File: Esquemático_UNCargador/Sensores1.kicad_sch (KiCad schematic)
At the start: 23 parts

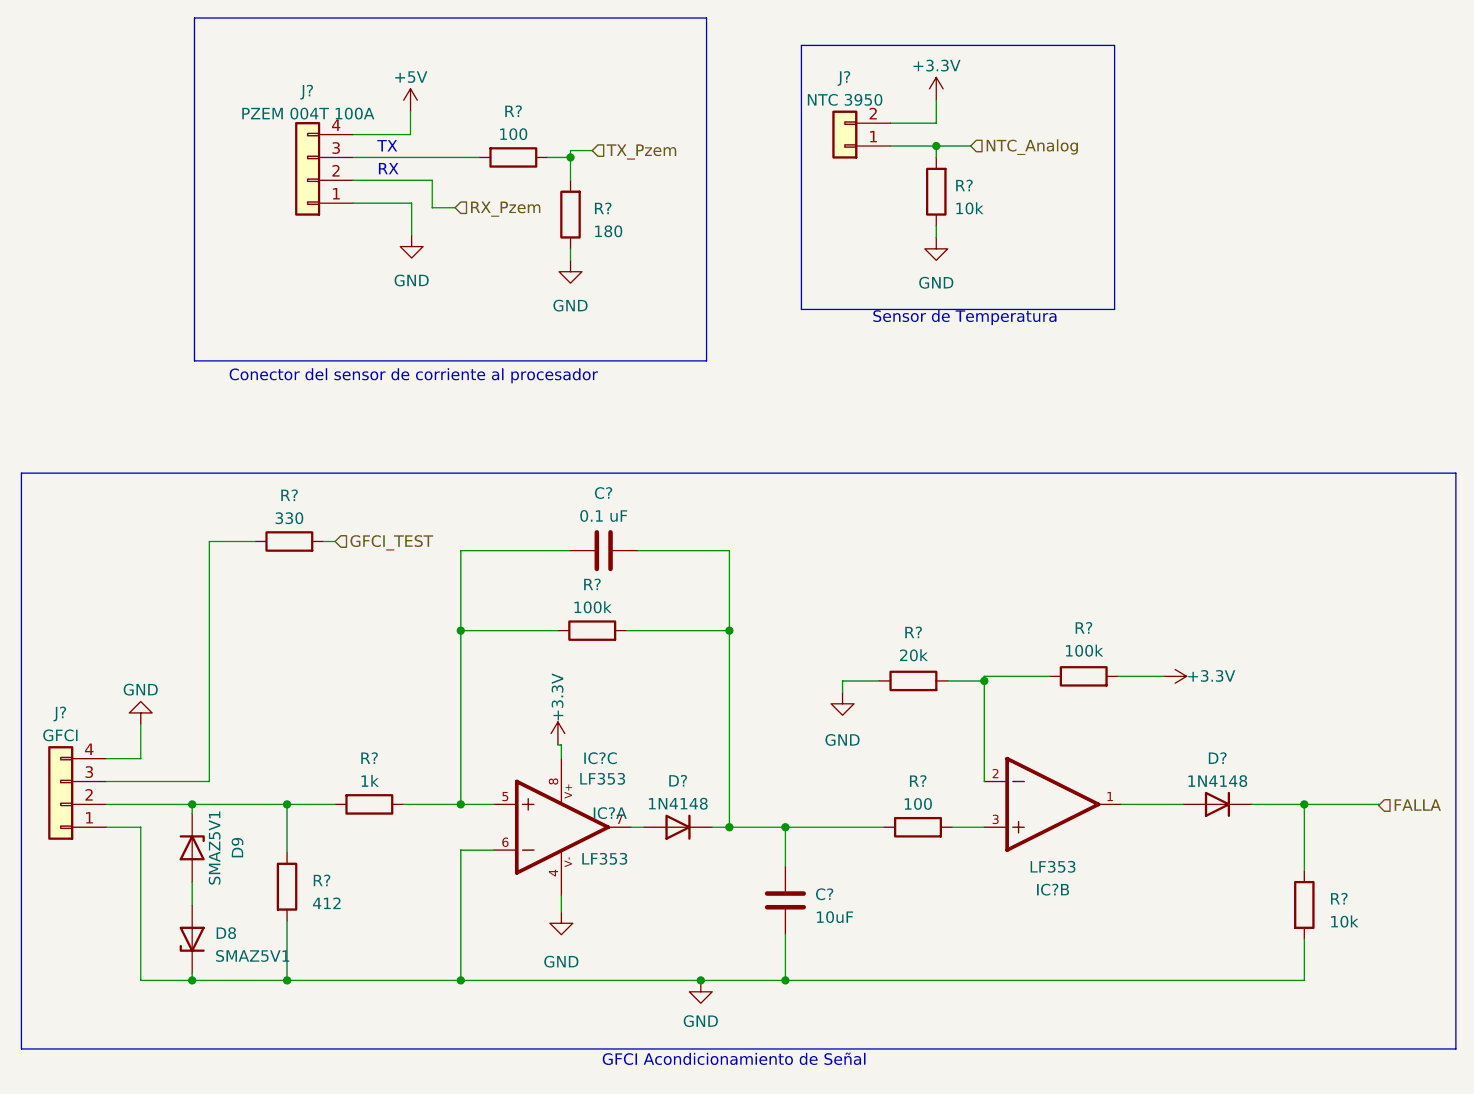
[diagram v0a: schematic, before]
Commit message: version inicial layout PCB
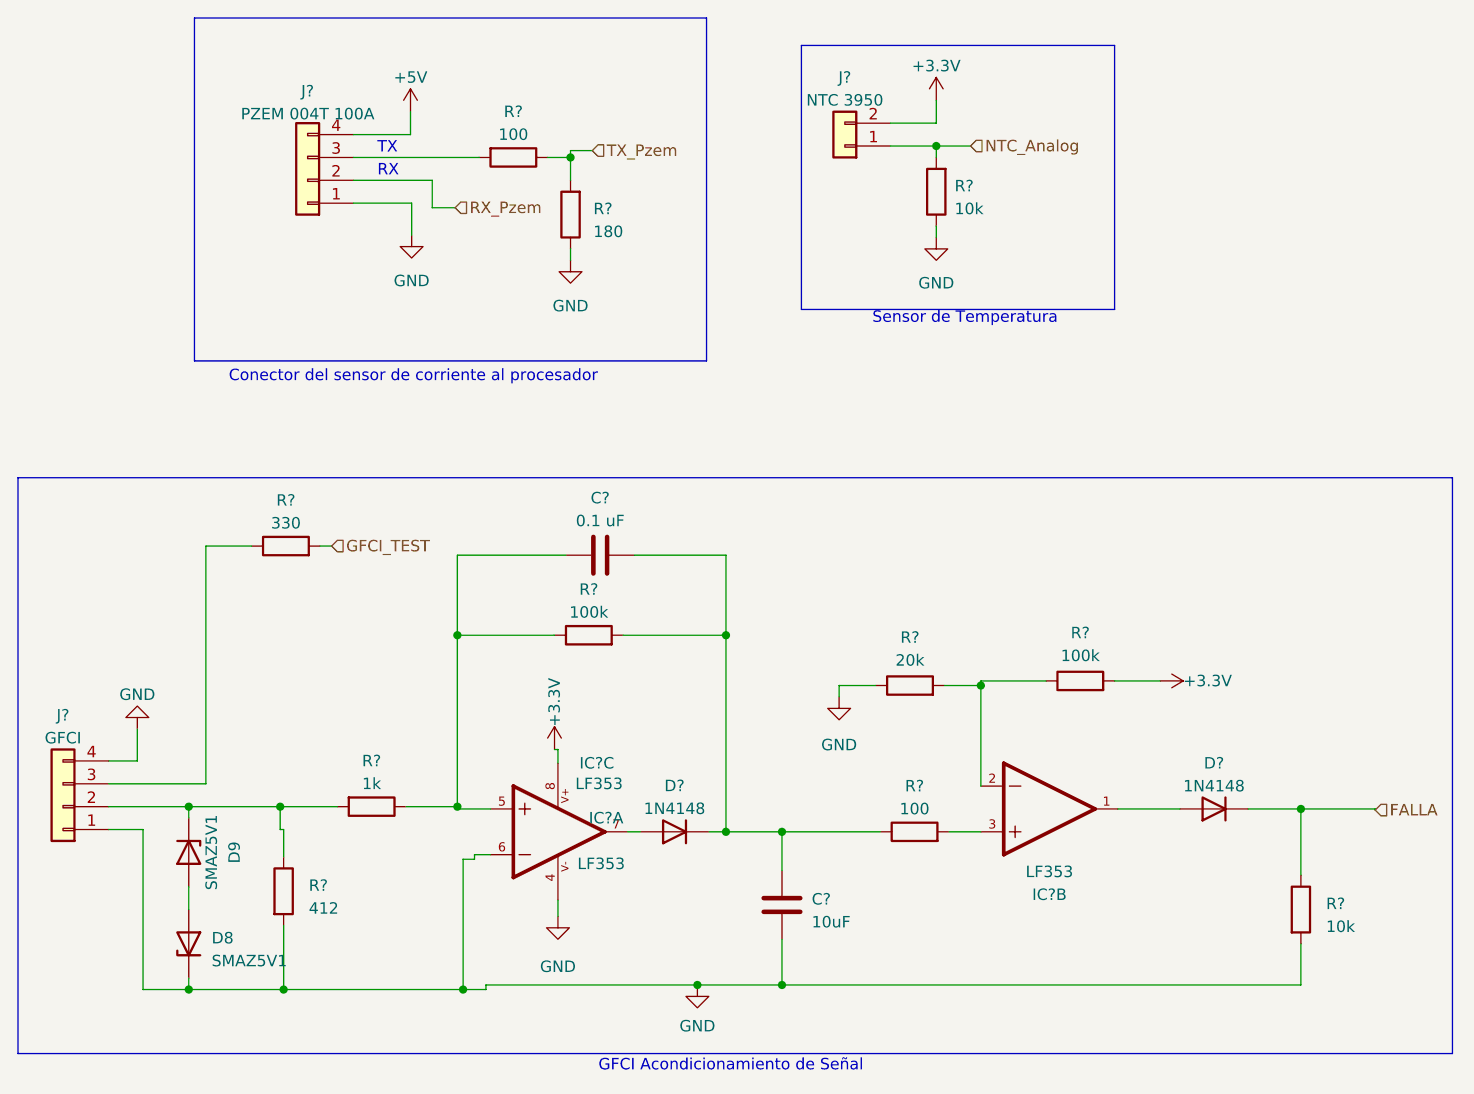
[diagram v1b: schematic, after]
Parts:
- D8, D9: footprint DO214AC:DO-214AC -> Esquemático_UNCargador:DO-214AC
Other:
- moved on the sheet: C?, D8, D9, D?, IC?A, IC?B, IC?C, R?
